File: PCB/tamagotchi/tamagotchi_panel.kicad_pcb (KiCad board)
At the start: 2 copper layers, 37.5 x 66 mm, 21 parts, among them J1 Programming port, J2 Conn_01x01_Female, J3 Conn_01x01_Female, J4 Conn_01x01_Male, J5 Conn_01x01_Male, SW1 Main Button, SW2 SW_Push, U1 ATtiny85V-10P, U2 OLED

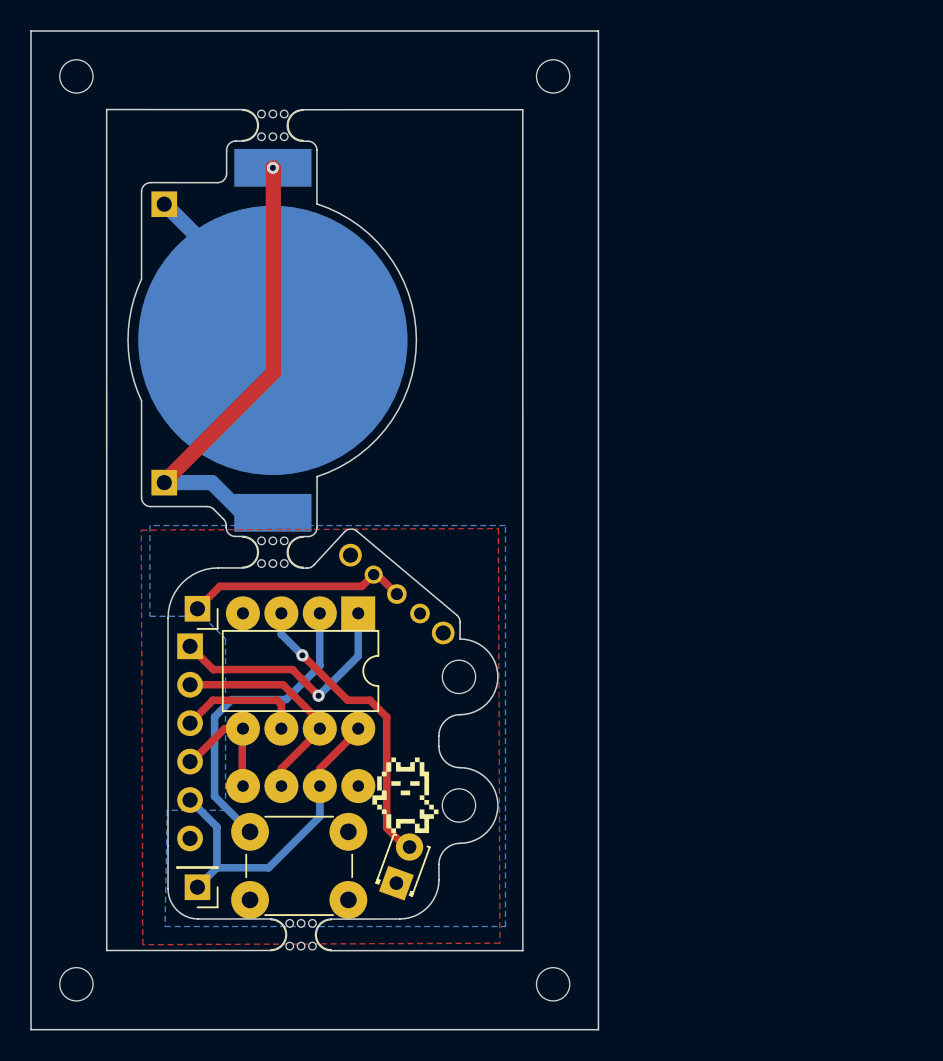
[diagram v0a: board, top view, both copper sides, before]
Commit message: optimized animation system
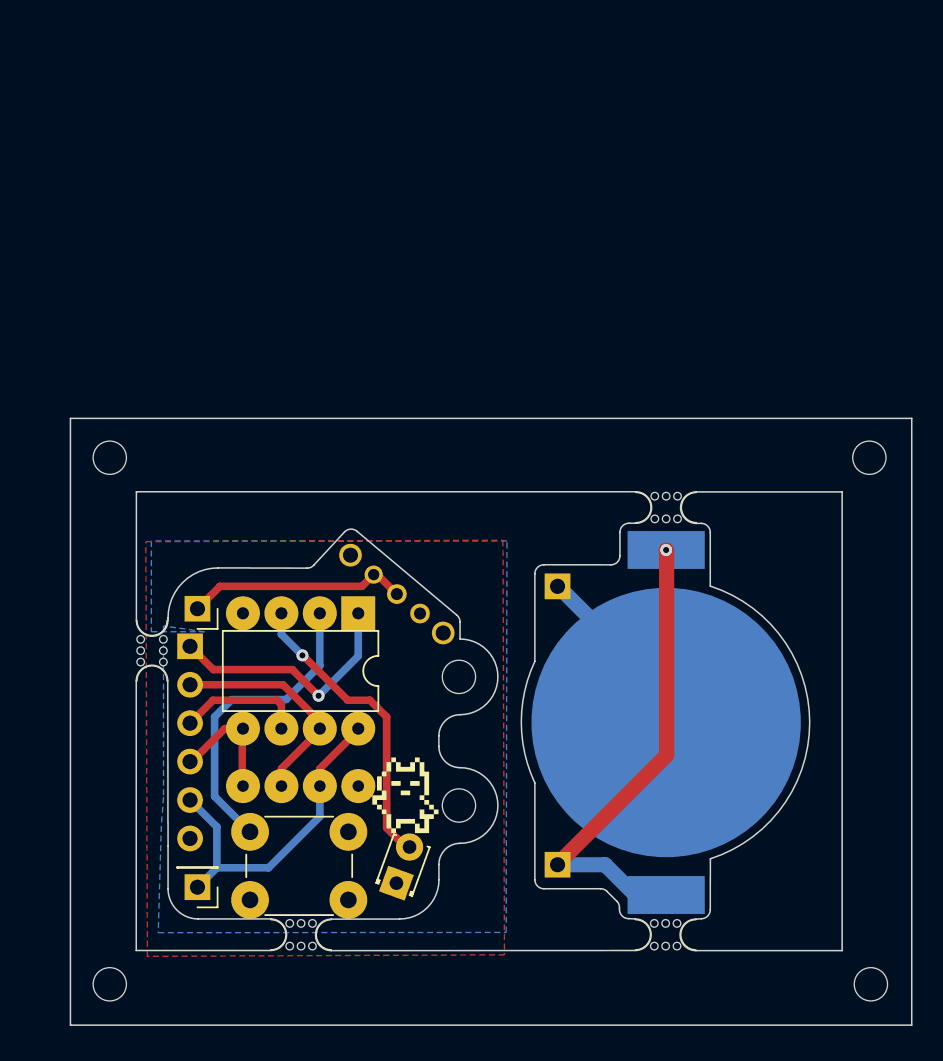
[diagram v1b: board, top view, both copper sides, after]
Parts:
- added mouse-bite-2mm-slot: VAL**, Panelization:mouse-bite-2mm-slot, F.Cu at (59.9, 73.2)
- moved BT2 36.2 mm to (60.0, 59.2)
- moved J5 36.2 mm to (52.8, 50.2)
- moved J4 36.2 mm to (52.8, 68.6)
- moved mouse-bite-2mm-slot 36.2 mm to (60.0, 45.0)
- moved H1 32.7 mm to (73.4, 41.7)
- moved H1 25.3 mm to (23.2, 41.7), turned to -90 degrees
- moved H1 21.0 mm to (73.5, 76.5), turned to -90 degrees
- moved mouse-bite-2mm-slot 10.3 mm to (26.0, 54.5), turned to 90 degrees
- moved H1 2.21 mm to (23.2, 76.5), turned to -90 degrees
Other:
- board size 37.5 x 66 mm -> 55.6 x 40.1 mm
